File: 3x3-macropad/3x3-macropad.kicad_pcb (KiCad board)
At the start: 2 copper layers, 38 parts, among them SW1 SW_Push, SW2 RotaryEncoder_Switch, U1 ATmega32U4-A, Y1 16MHz

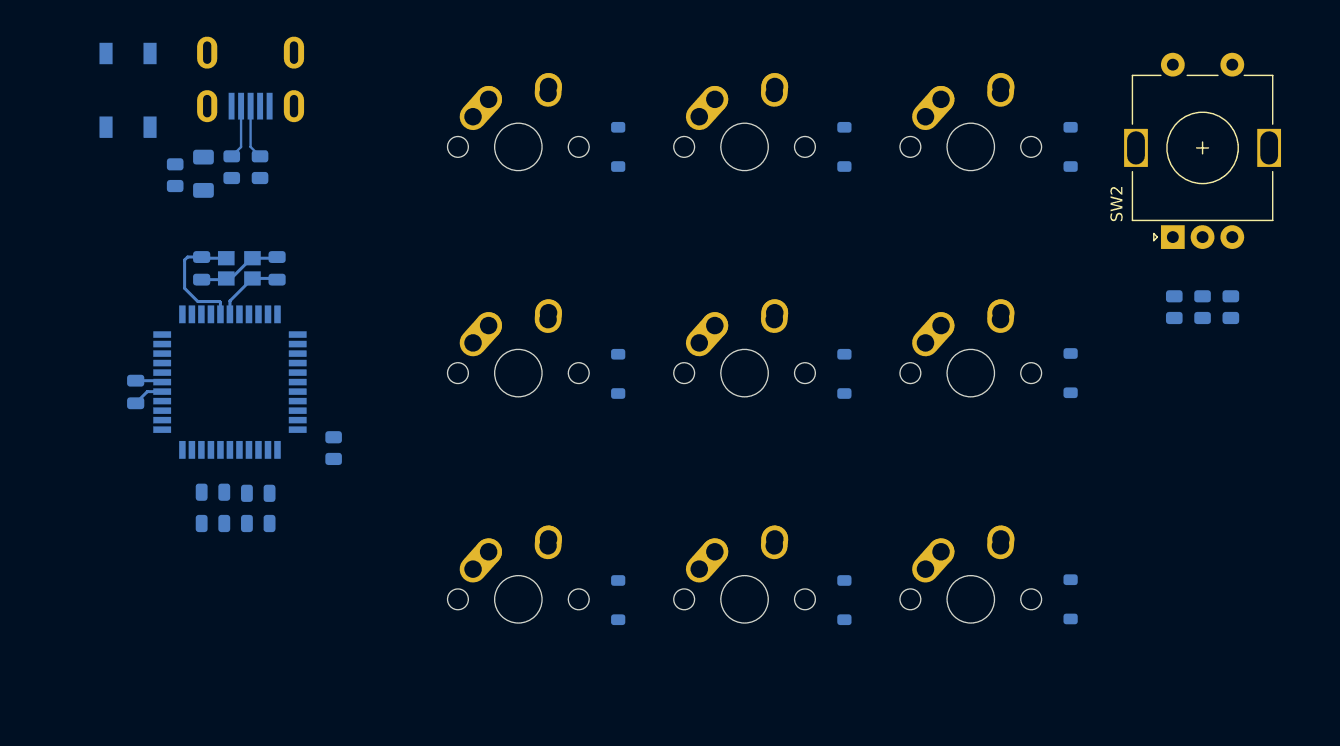
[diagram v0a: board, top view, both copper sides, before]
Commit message: first attempt routing 3x3
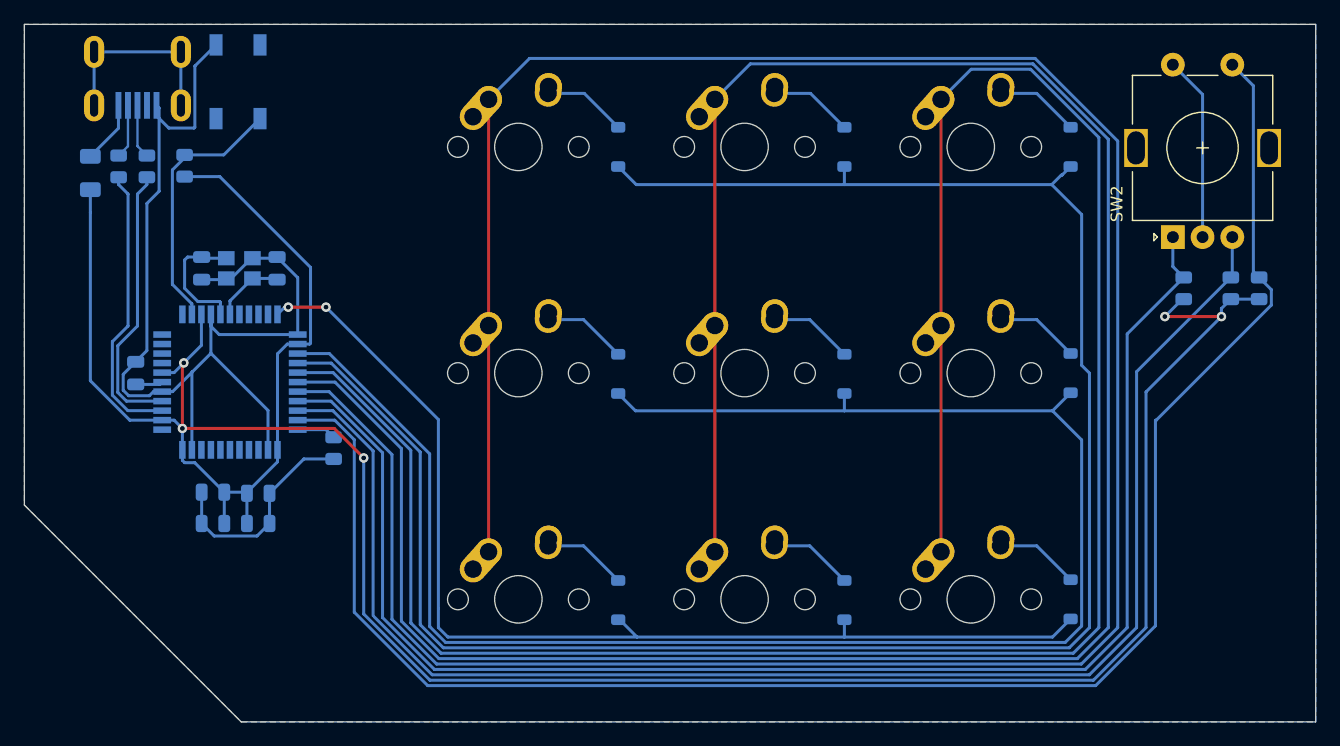
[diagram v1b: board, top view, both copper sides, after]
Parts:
- moved F1 9.51 mm to (150.6, 49.8)
- moved R2 9.51 mm to (155.4, 49.2)
- moved USB1 9.51 mm to (154.6, 39.6)
- moved R1 9.51 mm to (153.0, 49.2)
- moved SW1 9.28 mm to (163.0, 42.1)
- moved R5 7.31 mm to (248.9, 59.5)
- moved R6 2.24 mm to (242.6, 59.5)
- moved C6 1.59 mm to (154.4, 66.6), turned to 90 degrees
- moved R7 1.59 mm to (246.5, 59.5)
- moved R3 1.12 mm to (158.6, 49.2)
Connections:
- U1 pad 22: unconnected-(U1-PD5-Pad22) -> ROW2
- U1 pad 25: unconnected-(U1-PD4-Pad25) -> ROW1
- U1 pad 26: unconnected-(U1-PD6-Pad26) -> ROW0
- U1 pad 27: unconnected-(U1-PD7-Pad27) -> COL2
- U1 pad 28: unconnected-(U1-PB4-Pad28) -> COL1
- U1 pad 29: unconnected-(U1-PB5-Pad29) -> COL0
- U1 pad 30: unconnected-(U1-PB6-Pad30) -> ENCA
- U1 pad 31: unconnected-(U1-PC6-Pad31) -> ENCB
- U1 pad 32: unconnected-(U1-PC7-Pad32) -> ENCBTN
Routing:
- net +5V: track 0.00 -> 227.6 mm, vias 0 -> 5
- net COL0: track 0.00 -> 224.0 mm
- net COL1: track 0.00 -> 203.5 mm
- net COL2: track 0.00 -> 182.5 mm
- net ROW0: track 0.00 -> 165.1 mm
- net ROW1: track 0.00 -> 144.9 mm
- net ENCBTN: track 0.00 -> 144.6 mm
- net ENCB: track 0.00 -> 125.6 mm
- net ENCA: track 0.00 -> 123.9 mm
- net GND: track 9.76 -> 124.3 mm
- net ROW2: track 0.00 -> 93.0 mm, vias 0 -> 2
- net Net-(U1-D-): track 0.00 -> 23.9 mm
- net Net-(U1-D+): track 0.00 -> 23.2 mm
- net Net-(U1-~{RESET}): track 0.00 -> 22.1 mm
- net unconnected-(USB1-SHIELD-Pad6): track 0.00 -> 16.3 mm
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- added copper zone on B.Cu, net GND
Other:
- board outline added: 108.6 x 58.7 mm
